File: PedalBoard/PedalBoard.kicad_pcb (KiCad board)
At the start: 2 copper layers, 30 parts, among them U1 YAAJ_BluePill_Part_Like, U2 WM8731SEDS, U3 TL074, U4 MT3608

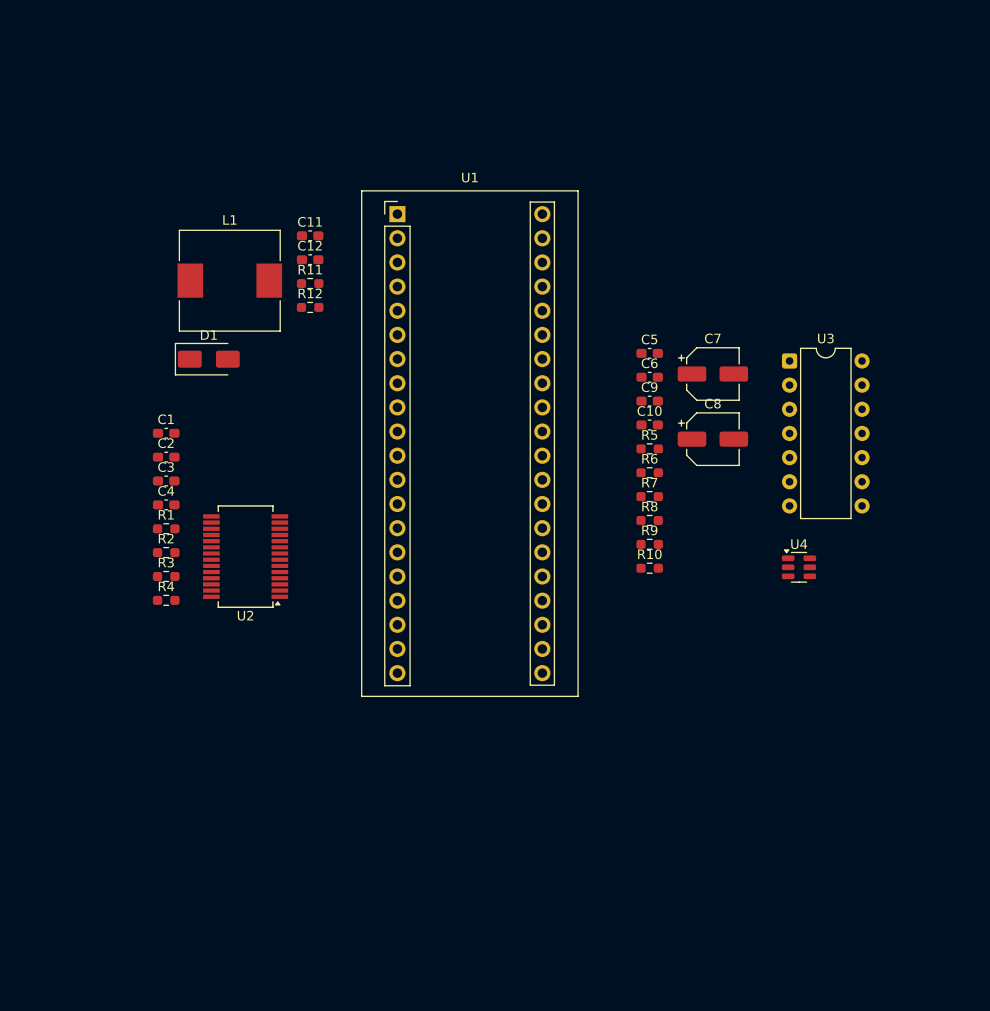
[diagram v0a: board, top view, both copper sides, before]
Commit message: згшщав
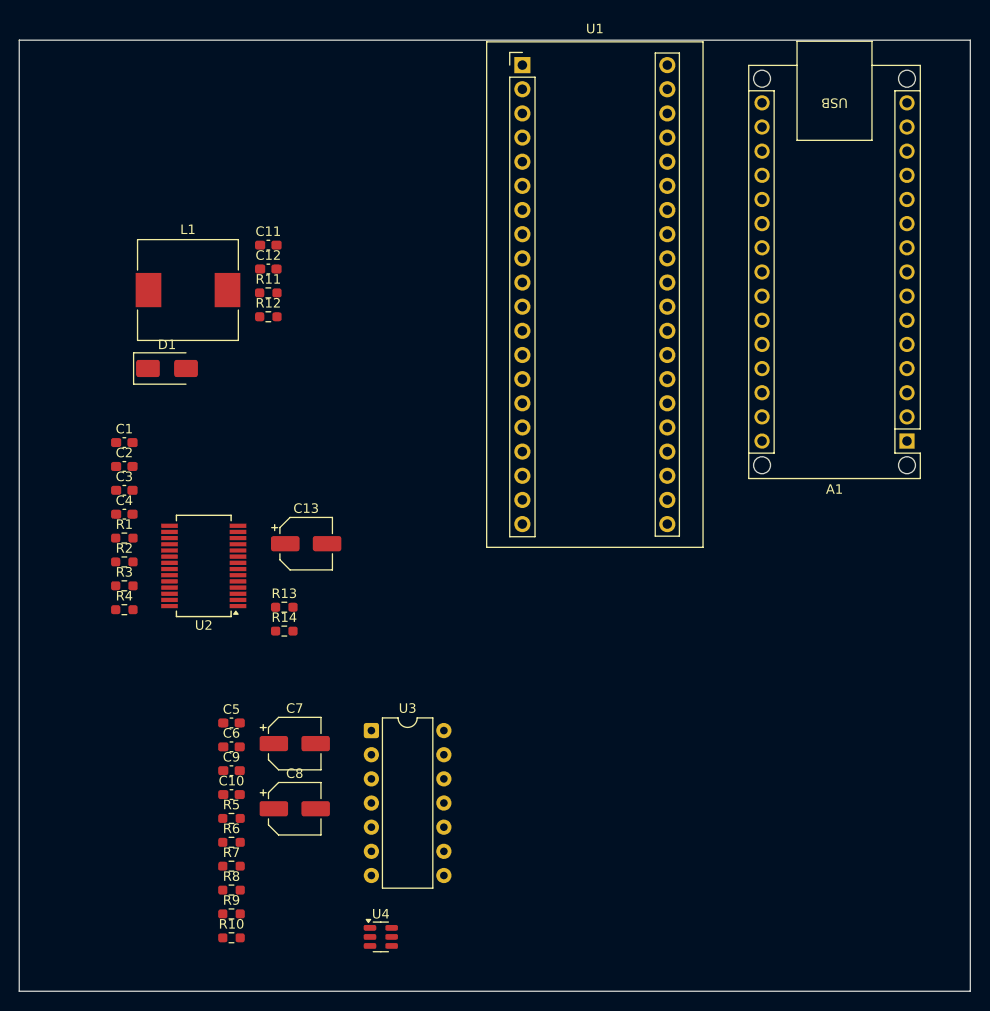
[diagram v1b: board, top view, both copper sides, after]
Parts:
- added A1: Arduino_Nano_ESP32, Module:Arduino_Nano_WithMountingHoles, F.Cu at (183.3, 102.2)
- added C13: 47uF 16V, Capacitor_SMD:CP_Elec_5x5.4, F.Cu at (120.2, 112.9)
- added R13: 10K, Resistor_SMD:R_0603_1608Metric_Pad0.98x0.95mm_HandSolder, F.Cu at (117.9, 119.6)
- added R14: 10K, Resistor_SMD:R_0603_1608Metric_Pad0.98x0.95mm_HandSolder, F.Cu at (117.9, 122.1)
- moved U4 58.7 mm to (128.0, 154.3)
- moved C6 58.7 mm to (112.3, 134.3)
- moved C7 58.7 mm to (119.0, 134.0)
- moved R5 58.7 mm to (112.3, 141.8)
- moved R8 58.7 mm to (112.3, 149.4)
- moved C10 58.7 mm to (112.3, 139.3)
- moved C8 58.7 mm to (119.0, 140.8)
- moved C9 58.7 mm to (112.3, 136.8)
- moved R10 58.7 mm to (112.3, 154.4)
- moved R6 58.7 mm to (112.3, 144.3)
- moved R7 58.7 mm to (112.3, 146.8)
- moved R9 58.7 mm to (112.3, 151.9)
- moved U3 58.7 mm to (127.0, 132.6)
- moved C5 58.7 mm to (112.3, 131.8)
- moved U1 20.5 mm to (142.9, 62.6)
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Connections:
- U3 pad 11: unconnected-(U3E-V--Pad11) -> GND
- U3 pad 12: unconnected-(U3D-+-Pad12) -> Net-(U3D-+)
- U3 pad 13: unconnected-(U3D---Pad13) -> Net-(U3D--)
- U3 pad 14: unconnected-(U3-Pad14) -> Net-(U3D--)
- U3 pad 4: unconnected-(U3E-V+-Pad4) -> +12V
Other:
- board outline added: 100 x 100 mm
